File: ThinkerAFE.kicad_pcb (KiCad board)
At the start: 4 copper layers, 29 x 41.2 mm, 57 parts, among them P1 CONN_01X10, P2 CONN_01X10, U1 TPS72325, U2 LM2664, U3 TLV70025DDC, U4 TPD4E1B06, U5 TPD4E1B06, U6 ADS1299, U7 TPD4E1B06

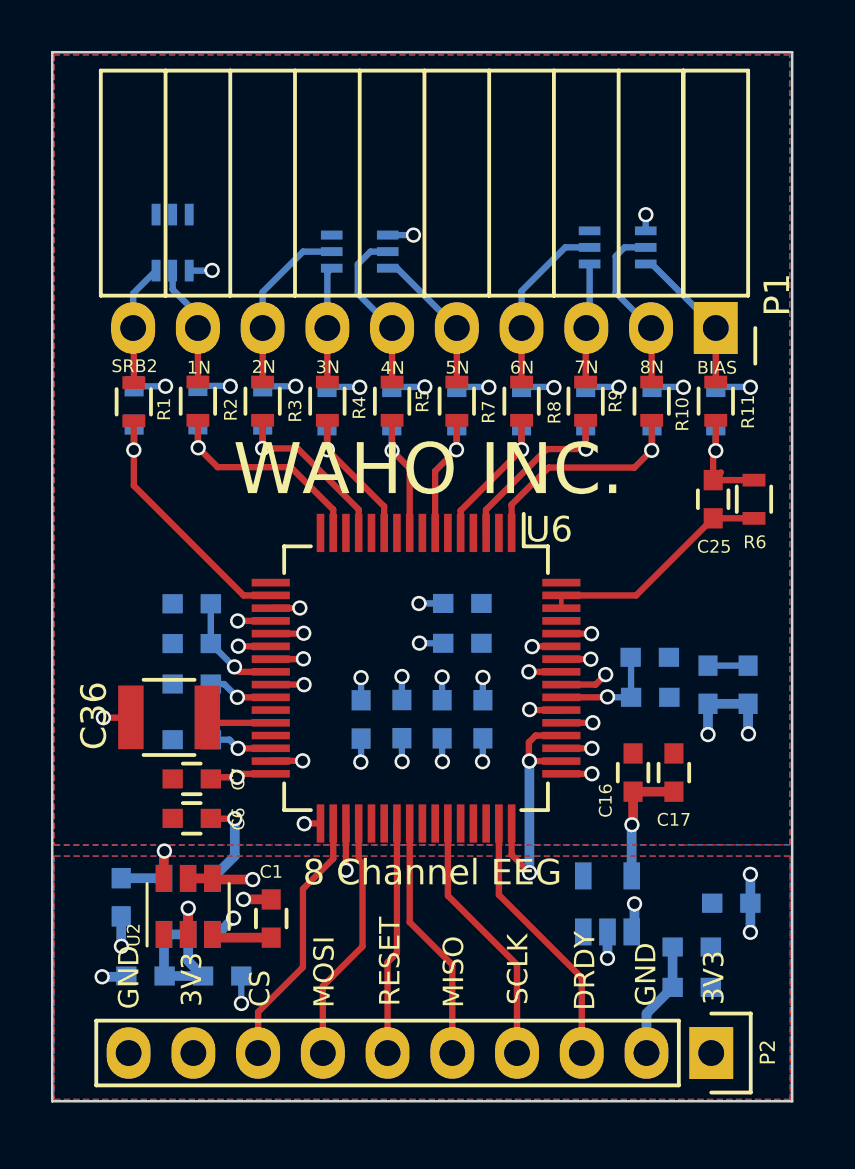
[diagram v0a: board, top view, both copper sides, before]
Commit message: Lots of progress with 0.1.0
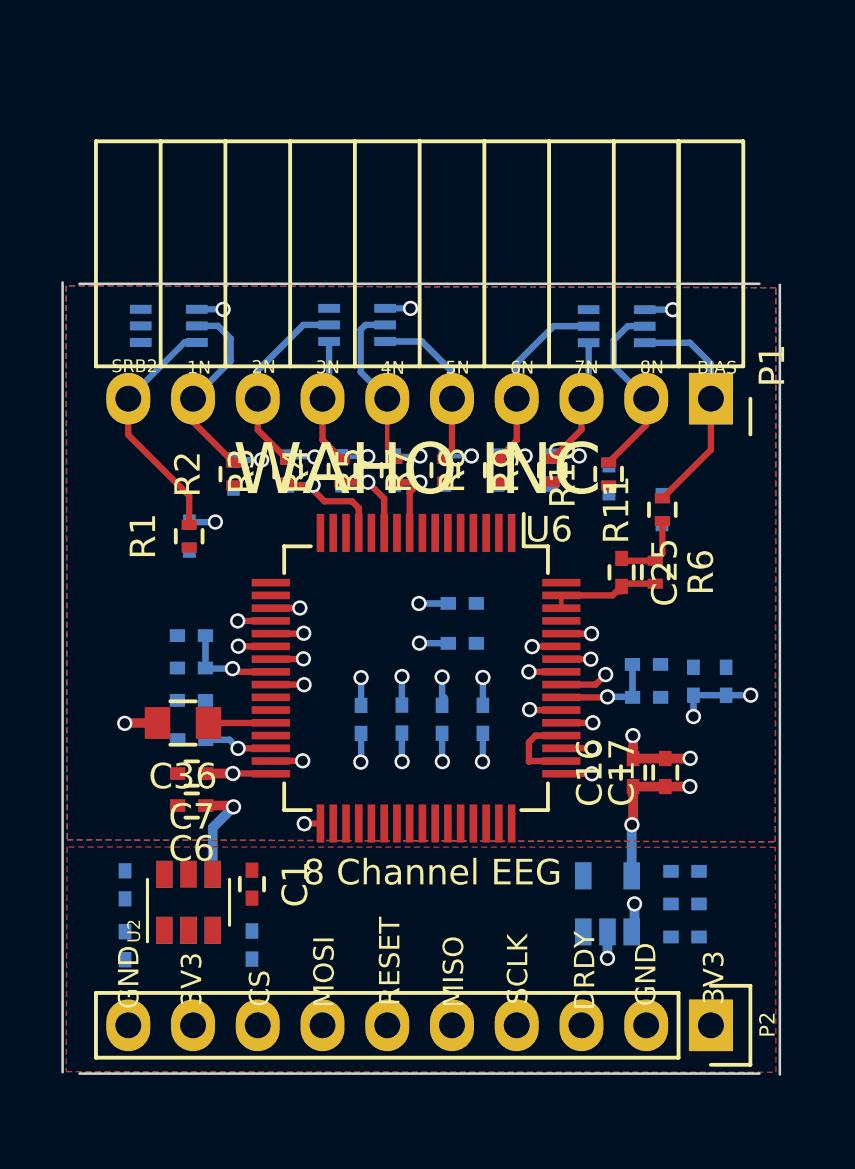
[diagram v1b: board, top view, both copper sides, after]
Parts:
- C1, C10, C11, C12, C13, C14, C15, C16, C17, C18, C19, C2, C20, C21, C22, C23, C24, C25, C26, C27, C28, C29, C3, C30, C31, C32, C33, C34, C35, C37, C4, C5, C6, C7, C8, C9: footprint Capacitors_SMD:C_0603 -> Capacitors_SMD:C_0402
- C36: footprint Capacitors_SMD:C_1210 -> Capacitors_SMD:C_0805
- R1, R10, R11, R2, R3, R4, R5, R6, R7, R8, R9: footprint Resistors_SMD:R_0603 -> Resistors_SMD:R_0402
- moved R1 5.71 mm to (37.5, 47.5)
- moved C20 5.57 mm to (37.5, 47.5)
- moved R6 4.82 mm to (55.8, 48.9)
- moved R11 4.75 mm to (56.0, 46.4)
- moved C25 4.60 mm to (54.4, 48.9)
- moved C28 4.58 mm to (56.0, 46.4)
- moved C31 3.32 mm to (53.9, 45.2)
- moved R10 3.32 mm to (53.9, 45.0)
- moved U5 3.27 mm to (36.7, 39.2), turned to 90 degrees
- moved R2 3.19 mm to (39.2, 45.0)
- moved U7 3.09 mm to (54.3, 39.2)
- moved C18 3.04 mm to (39.2, 45.0)
- moved R9 3.01 mm to (51.7, 44.9)
- moved R3 2.92 mm to (41.3, 44.9)
- moved U4 2.88 mm to (44.1, 39.2)
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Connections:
- U6 pad 10: Net-(U6-Pad10) -> VDDA
- U6 pad 12: Net-(U6-Pad12) -> VDDA
- U6 pad 14: Net-(U6-Pad14) -> VDDA
- U6 pad 16: Net-(U6-Pad16) -> VDDA
- U6 pad 2: Net-(U6-Pad2) -> VDDA
- U6 pad 4: Net-(U6-Pad4) -> VDDA
- U6 pad 41: Net-(U6-Pad41) -> GNDA
- U6 pad 6: Net-(U6-Pad6) -> VDDA
- U6 pad 8: Net-(U6-Pad8) -> VDDA
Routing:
- net GNDA: track 40.9 -> 28.0 mm, vias 31 -> 25
- net VDD: track 15.5 -> 4.49 mm, vias 5 -> 1
- net /INSRB2: track 10.7 -> 0.00 mm, vias 1 -> 0
- net /DRDY: track 10.4 -> 0.00 mm
- net /MOSI: track 10.2 -> 0.00 mm
- net /MISO: track 10.1 -> 0.00 mm
- net /RESET: track 9.71 -> 0.00 mm
- net /SCLK: track 9.70 -> 0.00 mm
- net /IN8N: track 9.68 -> 0.00 mm, vias 1 -> 0
- net /IN1N: track 9.25 -> 0.00 mm, vias 1 -> 0
- net /CS: track 9.16 -> 0.00 mm
- net /-RAW: track 8.03 -> 0.00 mm, vias 1 -> 0
- net /IN7N: track 7.92 -> 0.01 mm, vias 1 -> 0
- net /IN6N: track 6.39 -> 0.00 mm, vias 1 -> 0
- net Net-(C1-Pad1): track 6.06 -> 0.00 mm, vias 2 -> 0
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- removed copper zone on B.Cu, net VDD
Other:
- board size 29 x 41.2 mm -> 28.1 x 31.1 mm

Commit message: Lots of progress
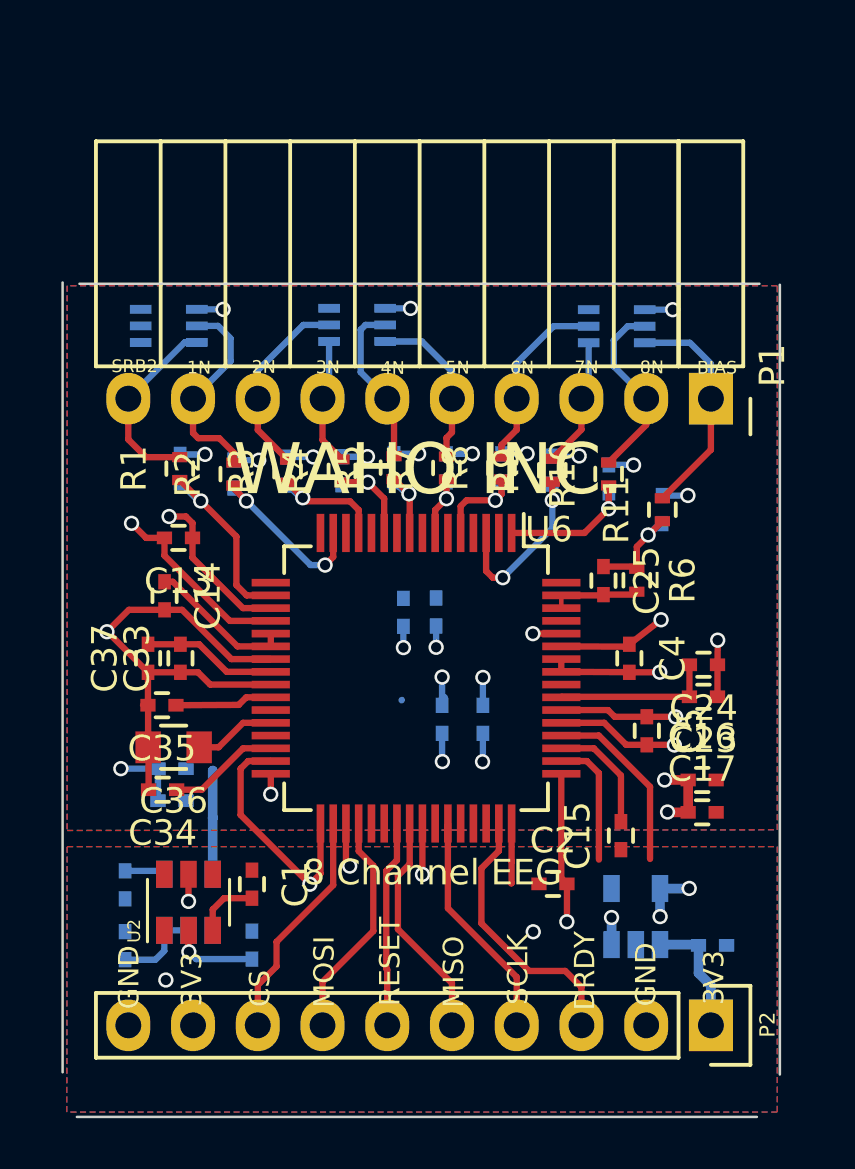
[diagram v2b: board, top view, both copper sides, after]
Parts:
- C13, C14, C15, C2, C23, C24, C33, C34, C35, C37, C4, C5: moved to F.Cu
- C6, C7: moved to B.Cu
- moved C27 11.7 mm to (47.2, 50.4)
- moved C26 11.7 mm to (45.9, 50.4)
- moved C13 11.3 mm to (37.1, 47.5), turned to 180 degrees
- moved C14 9.11 mm to (36.5, 49.8), turned to 270 degrees
- moved C5 8.80 mm to (55.4, 55.1), turned to 270 degrees
- moved C4 6.58 mm to (54.7, 52.3), turned to 270 degrees
- moved C2 5.24 mm to (51.8, 61.1), turned to 0 degrees
- moved C15 2.88 mm to (54.4, 59.2), turned to 90 degrees
- moved C16 2.73 mm to (57.6, 57.0), turned to 0 degrees
- moved C20 2.68 mm to (37.1, 44.8)
- moved R1 2.68 mm to (37.1, 44.8)
- moved C34 2.27 mm to (36.4, 57.4)
- moved C24 2.24 mm to (57.7, 52.5)
- moved C23 2.23 mm to (57.7, 53.8)
- moved C17 2.13 mm to (57.6, 58.3), turned to 0 degrees
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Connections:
- C13 pad 2: GNDA -> VSSA
- C14 pad 2: GNDA -> VSSA
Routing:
- net VDD: track 4.49 -> 35.0 mm, vias 1 -> 5
- net VSSA: track 15.5 -> 43.5 mm, vias 9 -> 6
- net GNDA: track 28.0 -> 42.6 mm, vias 25 -> 22
- net /DRDY: track 0.00 -> 10.7 mm
- net /MOSI: track 0.00 -> 9.15 mm
- net /MISO: track 0.00 -> 9.04 mm
- net /SCLK: track 0.00 -> 8.99 mm
- net /RESET: track 0.00 -> 8.98 mm
- net VDDA: track 19.2 -> 28.0 mm, vias 14 -> 9
- net /CS: track 0.00 -> 8.11 mm
- net /INSRB2: track 0.00 -> 7.78 mm, vias 0 -> 1
- net /-RAW: track 0.00 -> 7.74 mm, vias 0 -> 1
- net /IN7N: track 0.01 -> 7.47 mm, vias 0 -> 2
- net /IN1N: track 0.00 -> 7.19 mm, vias 0 -> 2
- net /IN8N: track 0.00 -> 5.74 mm, vias 0 -> 1
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- added copper zone on B.Cu, net GNDA
- added copper zone on F.Cu, net VDD
- removed copper zone on In1.Cu, net VDD
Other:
- board size 28.1 x 31.1 mm -> 28.1 x 32.7 mm
